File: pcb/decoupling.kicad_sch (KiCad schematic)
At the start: 24 parts

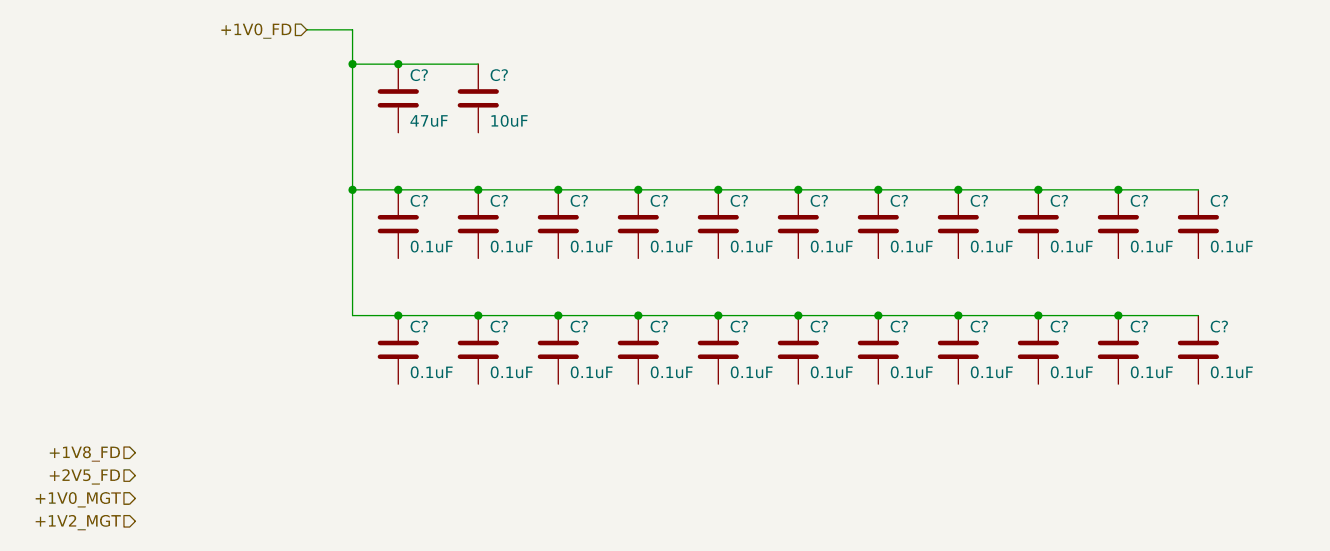
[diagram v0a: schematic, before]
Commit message: decoupling
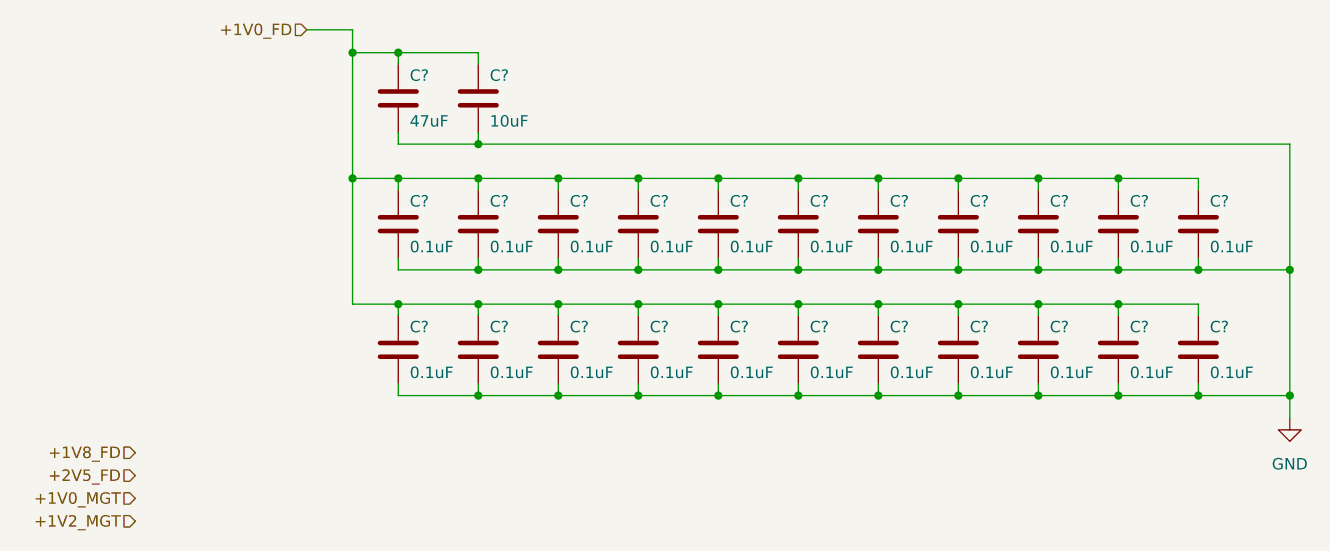
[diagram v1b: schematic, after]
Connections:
- net GND: now reaches C?.2
- net GND: now also C?.2, C?.2, C?.2, C?.2, C?.2, C?.2, C?.2, C?.2, C?.2, C?.2, C?.2, C?.2, C?.2, C?.2, C?.2, C?.2, C?.2, C?.2, C?.2, C?.2, C?.2, C?.2, C?.2
